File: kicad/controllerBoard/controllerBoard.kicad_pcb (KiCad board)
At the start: 2 copper layers, 150 x 150 mm, 763 parts, among them J1 Conn_02x20_Top_Bottom, J2 Conn_02x20_Top_Bottom, Q1 Q_PMOS_GSD, Q10 Q_NMOS_GSD, Q100 Q_NMOS_GSD, Q101 Q_PMOS_GSD, Q102 Q_NMOS_GSD, Q103 Q_PMOS_GSD, Q104 Q_NMOS_GSD, Q105 Q_PMOS_GSD, Q106 Q_NMOS_GSD, Q107 Q_PMOS_GSD, Q108 Q_NMOS_GSD, Q109 Q_PMOS_GSD, Q11 Q_PMOS_GSD, Q110 Q_NMOS_GSD, Q111 Q_PMOS_GSD, Q112 Q_NMOS_GSD, Q113 Q_PMOS_GSD, Q114 Q_NMOS_GSD, Q115 Q_PMOS_GSD, Q116 Q_NMOS_GSD, Q117 Q_PMOS_GSD, Q118 Q_NMOS_GSD, Q119 Q_PMOS_GSD, Q12 Q_NMOS_GSD, Q120 Q_NMOS_GSD, Q121 Q_PMOS_GSD, Q122 Q_NMOS_GSD, Q123 Q_PMOS_GSD, Q124 Q_NMOS_GSD, Q125 Q_PMOS_GSD, Q126 Q_NMOS_GSD, Q127 Q_PMOS_GSD, Q128 Q_NMOS_GSD, Q129 Q_PMOS_GSD, Q13 Q_PMOS_GSD, Q130 Q_NMOS_GSD, Q131 Q_PMOS_GSD, Q132 Q_NMOS_GSD, Q133 Q_PMOS_GSD, Q134 Q_NMOS_GSD, Q135 Q_PMOS_GSD, Q136 Q_NMOS_GSD, Q137 Q_PMOS_GSD, Q138 Q_NMOS_GSD, Q139 Q_PMOS_GSD, Q14 Q_PMOS_GSD, Q140 Q_NMOS_GSD, Q141 Q_PMOS_GSD, Q142 Q_NMOS_GSD, Q143 Q_PMOS_GSD, Q144 Q_NMOS_GSD, Q145 Q_PMOS_GSD, Q146 Q_NMOS_GSD, Q147 Q_PMOS_GSD, Q148 Q_NMOS_GSD, Q149 Q_PMOS_GSD, Q15 Q_PMOS_GSD, Q150 Q_NMOS_GSD, Q151 Q_PMOS_GSD, Q152 Q_NMOS_GSD, Q153 Q_PMOS_GSD, Q154 Q_NMOS_GSD, Q155 Q_PMOS_GSD, Q156 Q_NMOS_GSD, Q157 Q_PMOS_GSD, Q158 Q_NMOS_GSD, Q159 Q_PMOS_GSD, Q16 Q_NMOS_GSD, Q160 Q_NMOS_GSD, Q161 Q_PMOS_GSD, Q162 Q_NMOS_GSD, Q163 Q_PMOS_GSD, Q164 Q_NMOS_GSD, Q165 Q_PMOS_GSD, Q166 Q_NMOS_GSD, Q167 Q_PMOS_GSD, Q168 Q_NMOS_GSD, Q169 Q_PMOS_GSD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

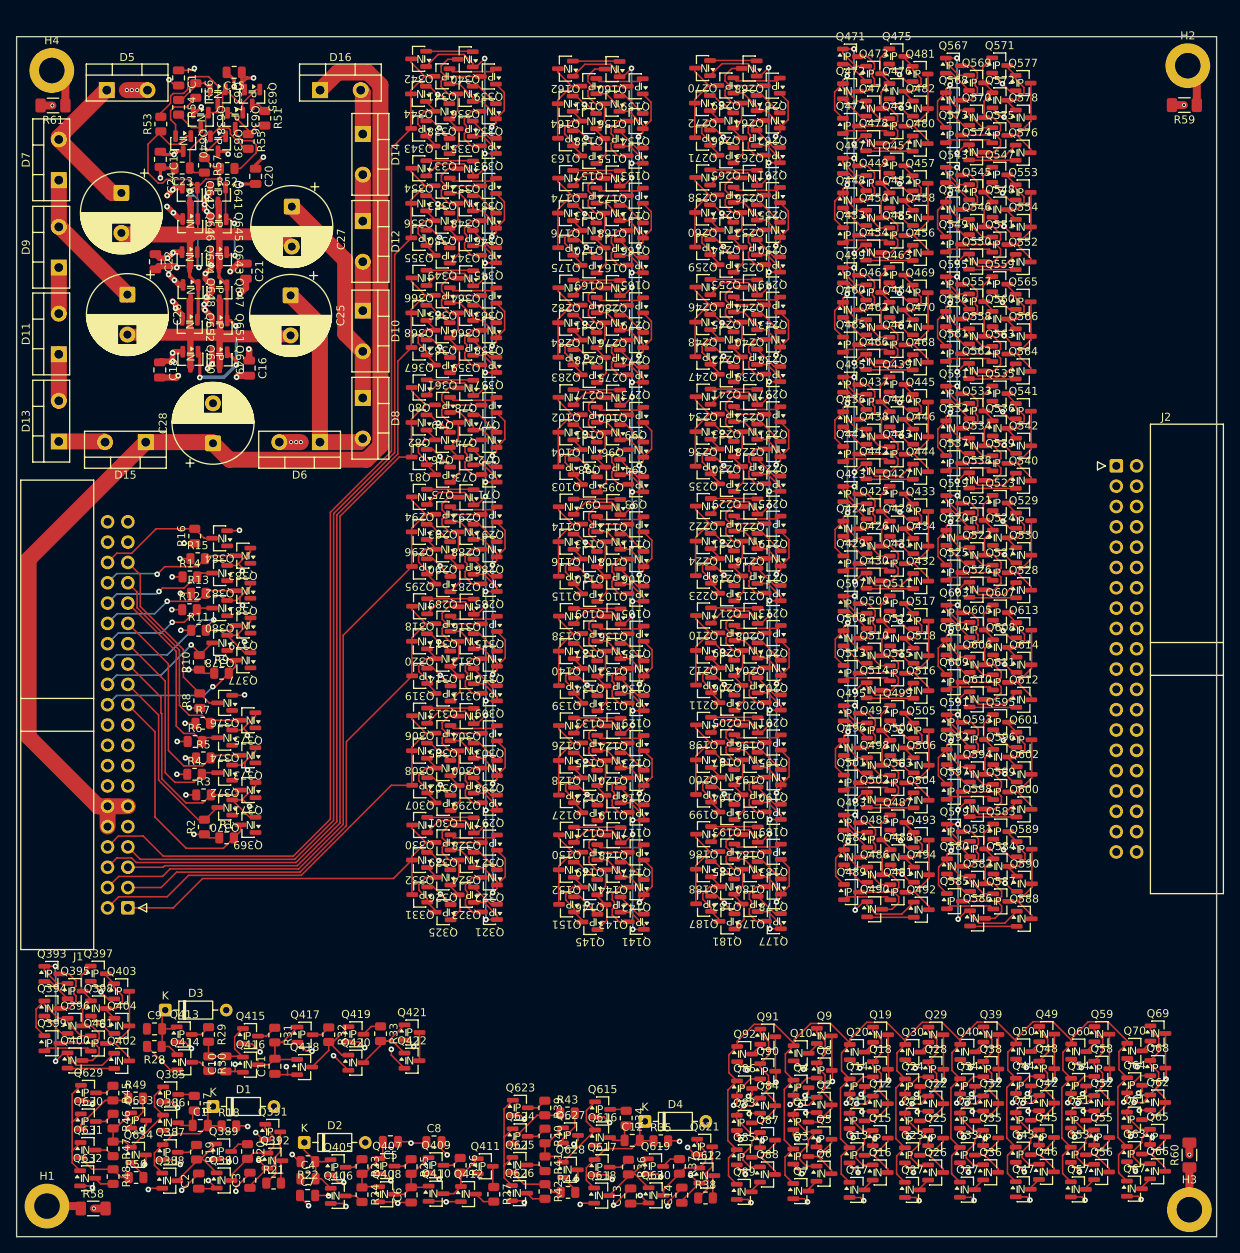
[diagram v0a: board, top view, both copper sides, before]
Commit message: routed data lines
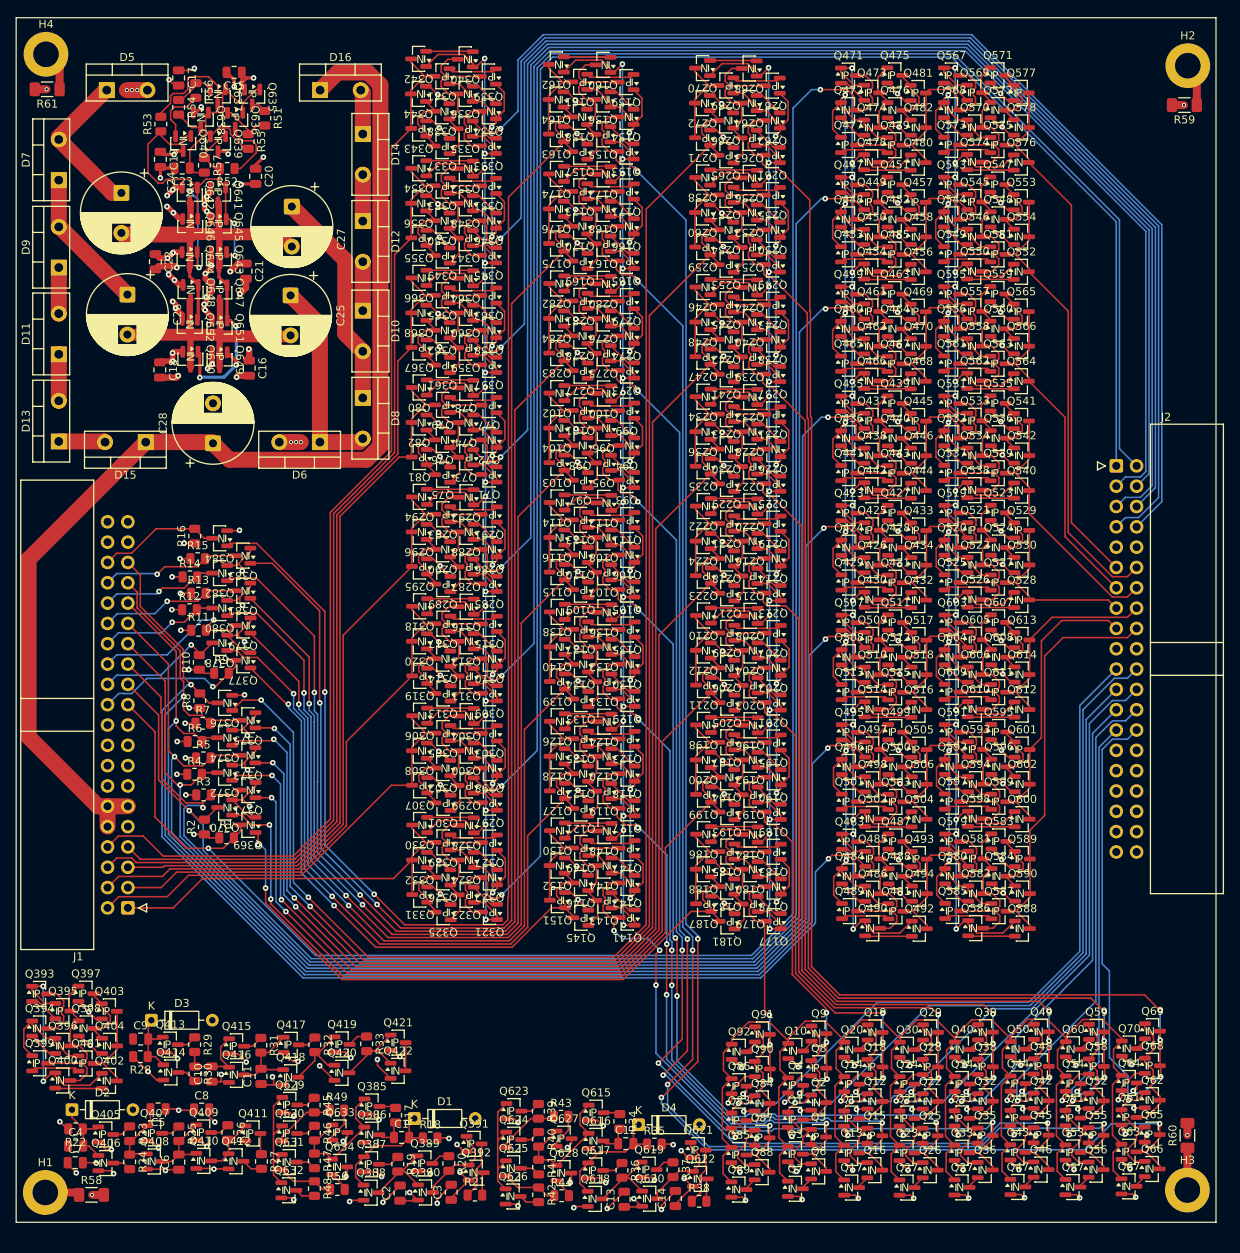
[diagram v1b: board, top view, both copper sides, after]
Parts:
- moved C5 29.3 mm to (50.6, 150.3)
- moved C6 29.3 mm to (53.2, 156.9)
- moved D2 29.3 mm to (39.8, 150.4)
- moved Q405 29.3 mm to (44.1, 153.5)
- moved Q406 29.3 mm to (44.2, 157.1)
- moved Q407 29.3 mm to (50.2, 153.3)
- moved Q410 29.3 mm to (56.4, 156.8)
- moved R22 29.3 mm to (40.3, 152.8)
- moved R25 29.3 mm to (53.2, 153.4)
- moved R27 29.3 mm to (63.5, 156.8)
- moved C4 29.3 mm to (40.3, 154.9)
- moved C7 29.3 mm to (40.3, 157.0)
- moved C8 29.3 mm to (56.1, 150.3)
- moved Q408 29.3 mm to (50.2, 156.8)
- moved Q409 29.3 mm to (56.4, 153.2)
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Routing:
- net /Addr_{in}_{0}: track 7.65 -> 229.1 mm, vias 0 -> 1
- net /Addr_{in}_{1}: track 7.65 -> 217.6 mm, vias 0 -> 1
- net /Addr_{in}_{2}: track 7.65 -> 211.3 mm, vias 0 -> 1
- net /~{BL}_{nctrl ncl 7}: track 14.6 -> 207.9 mm, vias 0 -> 4
- net /BL_{0}: track 37.1 -> 229.3 mm, vias 0 -> 2
- net /Addr_{in}_{3}: track 7.65 -> 196.8 mm, vias 0 -> 1
- net /BL_{1}: track 31.2 -> 216.1 mm, vias 0 -> 2
- net /Addr_{in}_{4}: track 7.65 -> 189.1 mm, vias 0 -> 1
- net /BL_{ctrl cl 7}: track 8.43 -> 187.4 mm, vias 0 -> 2
- net /BL_{2}: track 35.5 -> 211.4 mm, vias 0 -> 2
- net /~{BL}_{ctrl cl 7}: track 8.43 -> 180.9 mm, vias 0 -> 2
- net /~{BL}_{nctrl ncl 6}: track 14.6 -> 185.6 mm, vias 0 -> 4
- net /Addr_{in}_{5}: track 7.65 -> 174.6 mm, vias 0 -> 1
- net /BL_{3}: track 33.2 -> 197.1 mm, vias 0 -> 2
- net /BL_{ctrl cl 6}: track 8.43 -> 169.0 mm, vias 0 -> 2
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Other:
- board size 150 x 150 mm -> 150 x 150.6 mm
- copper layers 2 -> 4
